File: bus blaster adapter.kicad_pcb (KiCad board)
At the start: 2 copper layers, 50 x 50 mm, 72 parts, among them P101 CONN_02X10, P102 CONN_02X10

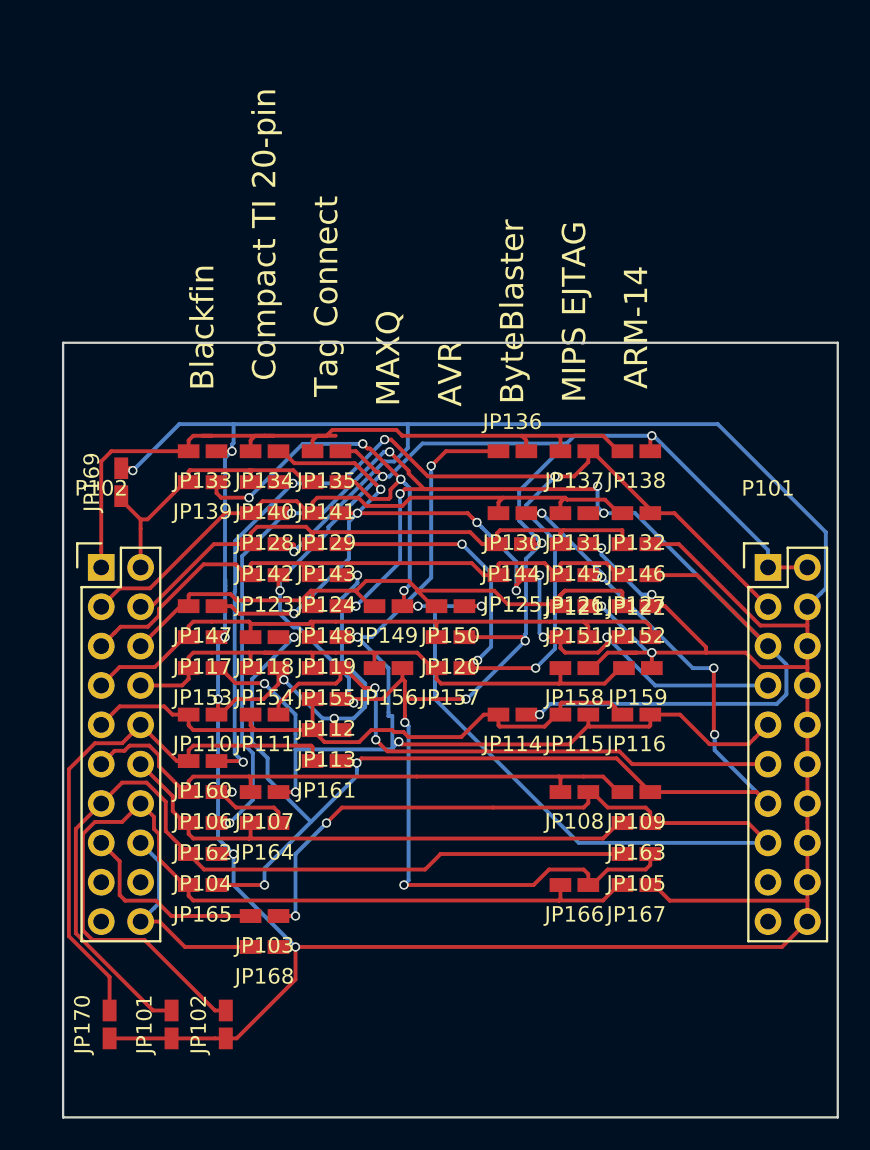
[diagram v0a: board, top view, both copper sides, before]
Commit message: Layout work, could probably use double checking...
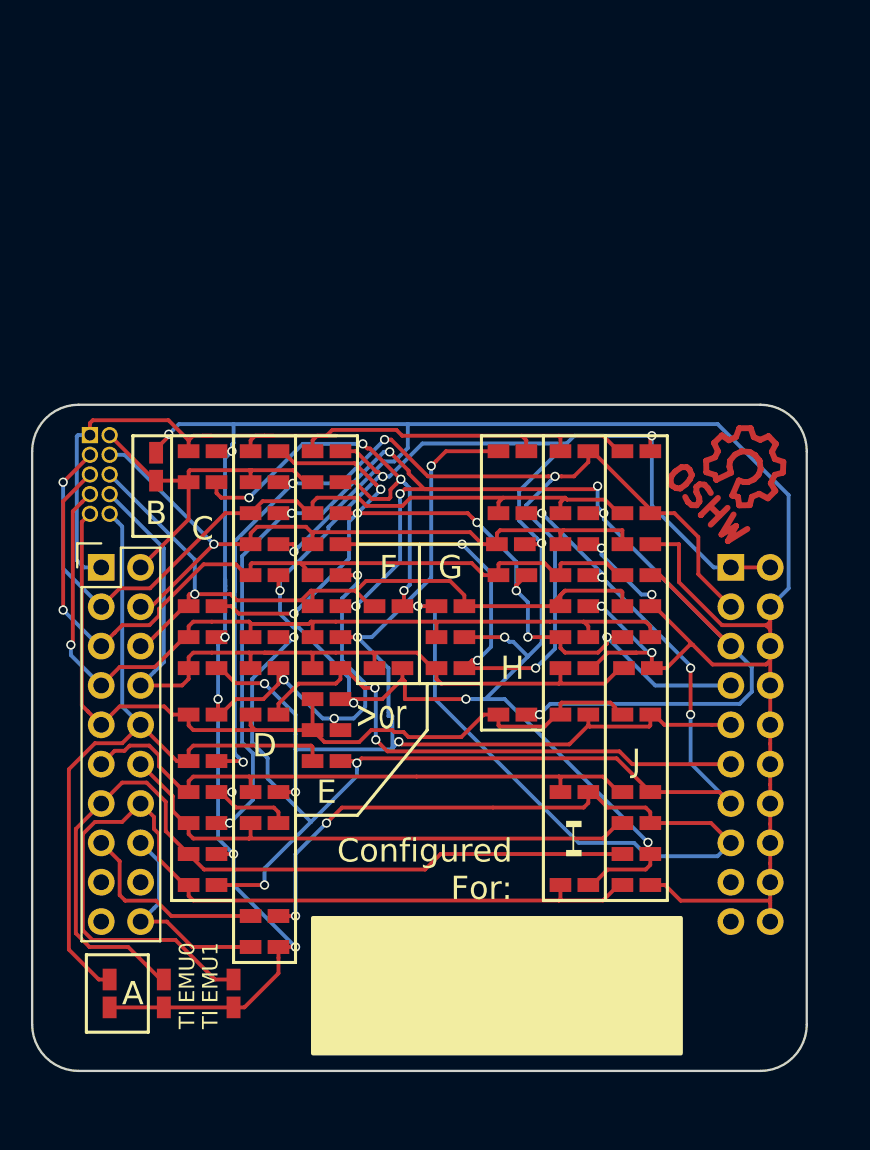
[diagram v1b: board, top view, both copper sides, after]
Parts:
- added P103: CONN_02X05, header_1:10pin_1.27pitch, F.Cu at (102.4, 108.5)
- added REF**: Symbol_OSHW-Logo_CopperTop, Symbols:Symbol_OSHW-Logo_CopperTop, F.Cu at (144.0, 108.0)
- moved JP169 2.46 mm to (106.0, 108.0)
- moved P101 2.40 mm to (143.1, 114.5)
- moved JP101 2.06 mm to (106.5, 142.0)
- moved JP102 2.06 mm to (111.0, 142.0)
- moved JP170 2.00 mm to (103.0, 142.0)
- turned JP150 to 0 degrees
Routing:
- net GND: track 268.3 -> 223.4 mm
- net Net-(JP153-Pad2): track 39.3 -> 53.7 mm
- net Net-(JP110-Pad2): track 41.7 -> 56.1 mm
- net Net-(JP117-Pad2): track 42.8 -> 56.3 mm, vias 0 -> 1
- net Net-(JP123-Pad2): track 40.8 -> 53.7 mm, vias 0 -> 1
- net Net-(JP160-Pad2): track 36.3 -> 49.2 mm
- net Net-(JP128-Pad2): track 40.7 -> 52.3 mm, vias 0 -> 1
- net Net-(JP147-Pad2): track 41.0 -> 51.2 mm, vias 0 -> 1
- net Net-(JP142-Pad2): track 37.6 -> 46.7 mm, vias 0 -> 1
- net /VTREF: track 126.1 -> 118.1 mm, vias 9 -> 8
- net /TDI: track 105.8 -> 99.0 mm
- net /TSRST: track 106.1 -> 100.1 mm, vias 8 -> 7
- net Net-(JP133-Pad2): track 50.0 -> 55.6 mm
- net Net-(JP139-Pad2): track 19.5 -> 23.7 mm
- net /TDO: track 85.6 -> 81.4 mm
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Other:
- board size 50 x 50 mm -> 50 x 43 mm
- board text added: "14 20 10 10 10 10 14 14"
- board text added: ">or"
- board text added: "A"
- board text added: "B"
- board text added: "Blackfin Compact TI Tag Connect Maxim MAXQ AVR ByteBlaster MIPS EJTAG ARM-14"
- board text added: "C"
- board text added: "C A D E A B F H A B G H A B H A B I A B J"
- board text added: "Configured For:"
- board text added: "D"
- board text added: "E"
- board text added: "F"
- board text added: "G"
- board text added: "H"
- board text added: "Host"
- board text added: "Ian Rees - July 2016 - v1"
- board text added: "J"
- board text added: "Jumper Sections"
- board text added: "TI EMU0"
- board text added: "TI EMU1"
- board text added: "Target"
- board text added: "Target Pins Used"
- board text added: "github.com/ianrrees/busblaster-adapter"
- board text removed: "ARM-14"
- board text removed: "AVR"
- board text removed: "Blackfin"
- board text removed: "ByteBlaster"
- board text removed: "Compact TI 20-pin"
- board text removed: "MAXQ"
- board text removed: "MIPS EJTAG"
- board text removed: "Tag Connect"
